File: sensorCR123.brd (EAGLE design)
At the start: 29.3 x 16.2 mm, 21 parts, among them IC1 LM75AD, IC4 RFM69, X1 16 MHz

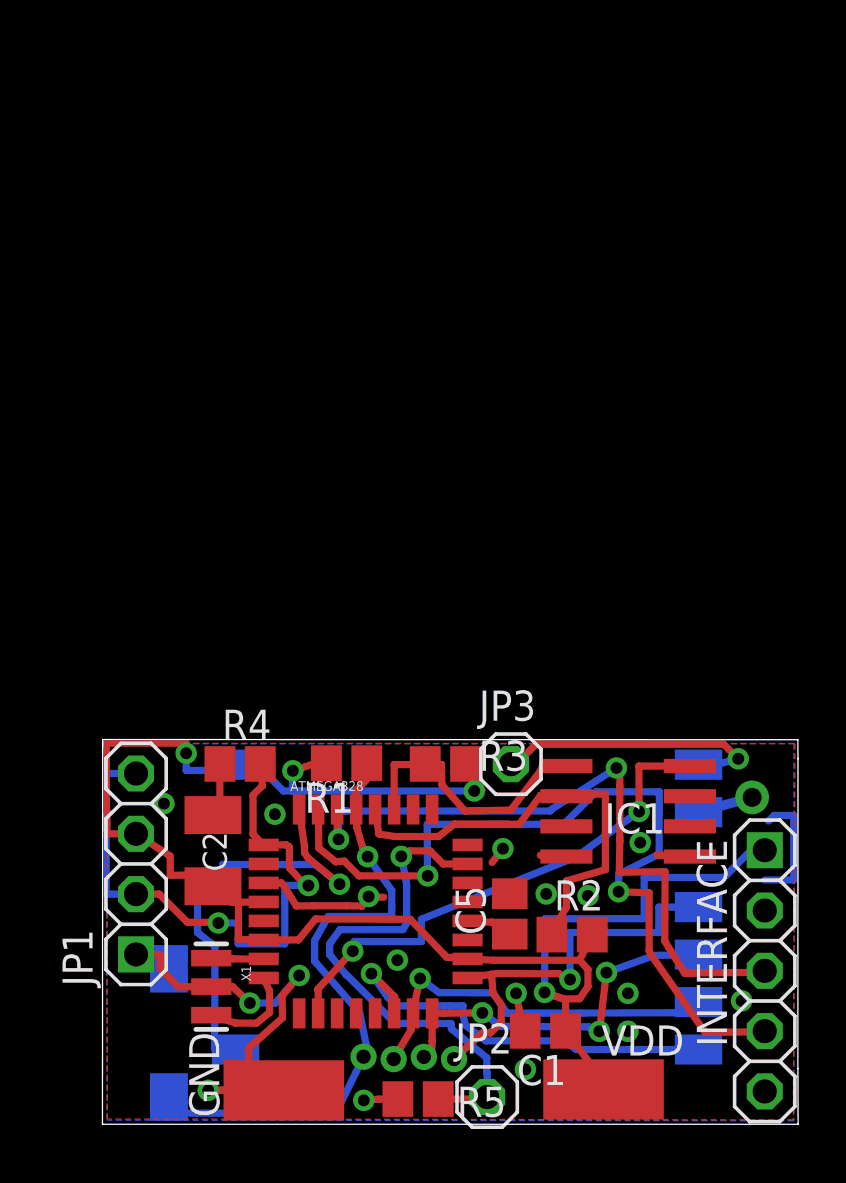
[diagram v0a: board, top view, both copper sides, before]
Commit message: Fixed bugs
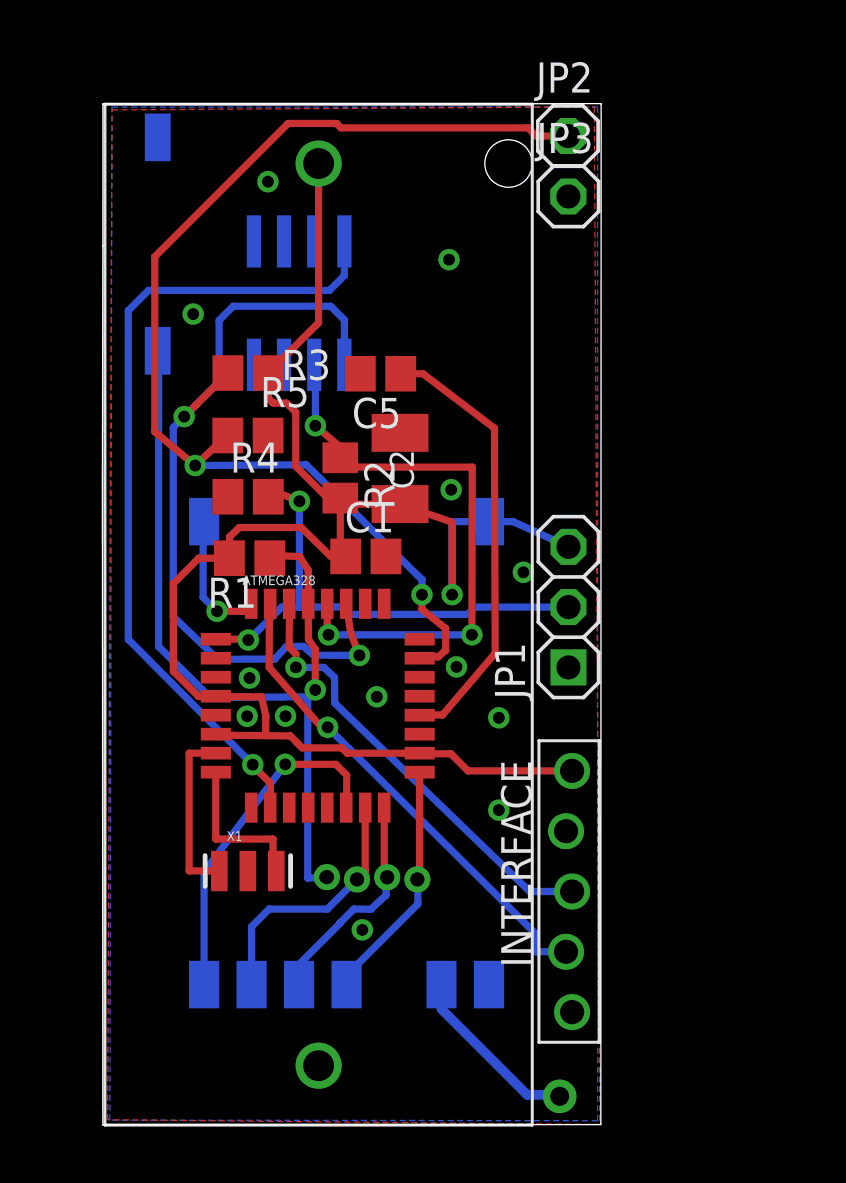
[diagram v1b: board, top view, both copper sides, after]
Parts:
- removed GND, VDD: (no value), wirepad:SMD2,54-5,08
- added U$3: BATT-CR123A, eagle-library-edeca.net-v5:KEYSTONE-2/3A
- INTERFACE: value (none) -> PINHD1X5SQUARE; device pinhead-2:1X05-S -> eagle-library-edeca.net-v5:PINHD1X05-SQUARE
- JP1: device pinhead-2:1X04-S -> pinhead-2:1X03-S
- RESET: device switch-tact:DTSM-3 -> smd-special:SMS-001
- moved JP2 40.6 mm to (19.6, 41.6)
- moved RESET 33.2 mm to (2.32, 37.1), turned to 0 degrees
- moved R5 28.9 mm to (6.12, 29.0), turned to 180 degrees
- moved IC1 25.5 mm to (8.27, 34.6), flipped to the bottom, turned to 0 degrees
- moved JP3 24.0 mm to (19.6, 39.1)
- moved C5 23.4 mm to (11.7, 31.6), turned to 180 degrees
- moved R2 21.6 mm to (10.0, 27.2), turned to 270 degrees
- moved C1 21.4 mm to (11.1, 23.9), turned to 0 degrees
- moved JP1 21.2 mm to (19.6, 21.8)
- moved R3 18.4 mm to (6.13, 31.6)
- moved C2 17.9 mm to (12.5, 27.6)
- moved U$1 15.0 mm to (19.3, 1.17)
- moved R4 11.3 mm to (6.13, 26.4)
- moved IC4 9.70 mm to (9.27, 13.9), turned to 270 degrees
- moved R1 9.55 mm to (6.19, 23.8)
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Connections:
- net D3: no longer JP1.4
- net GND: now also U$3.-VE; no longer GND.1
- net VCC: now also U$3.+VE; no longer VDD.1
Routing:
- net GND: track 52.7 -> 0.00 mm, vias 18 -> 13
- net A0: track 22.4 -> 47.6 mm, vias 1 -> 2
- net A4_SDA: track 12.4 -> 34.7 mm, vias 0 -> 2
- net AREF: track 2.09 -> 18.6 mm
- net D1_TX: track 34.9 -> 20.7 mm, vias 2 -> 1
- net D2: track 19.1 -> 5.61 mm
- net D6: track 21.7 -> 35.0 mm, vias 2 -> 1
- net D0_RX: track 29.6 -> 18.9 mm, vias 2 -> 1
- net RST: track 27.4 -> 35.8 mm, vias 1 -> 2
- net D13_SCK: track 17.6 -> 10.2 mm, vias 1 -> 0
- net VCC: track 77.2 -> 70.0 mm, vias 4 -> 1
- net D12_MISO: track 15.8 -> 9.55 mm, vias 3 -> 0
- net D11_MOSI: track 16.1 -> 10.9 mm, vias 1 -> 0
- net N$3: track 2.34 -> 7.53 mm
- net N$1: track 2.23 -> 7.36 mm
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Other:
- board size 29.3 x 16.2 mm -> 21 x 43 mm

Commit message: aaa
aaa
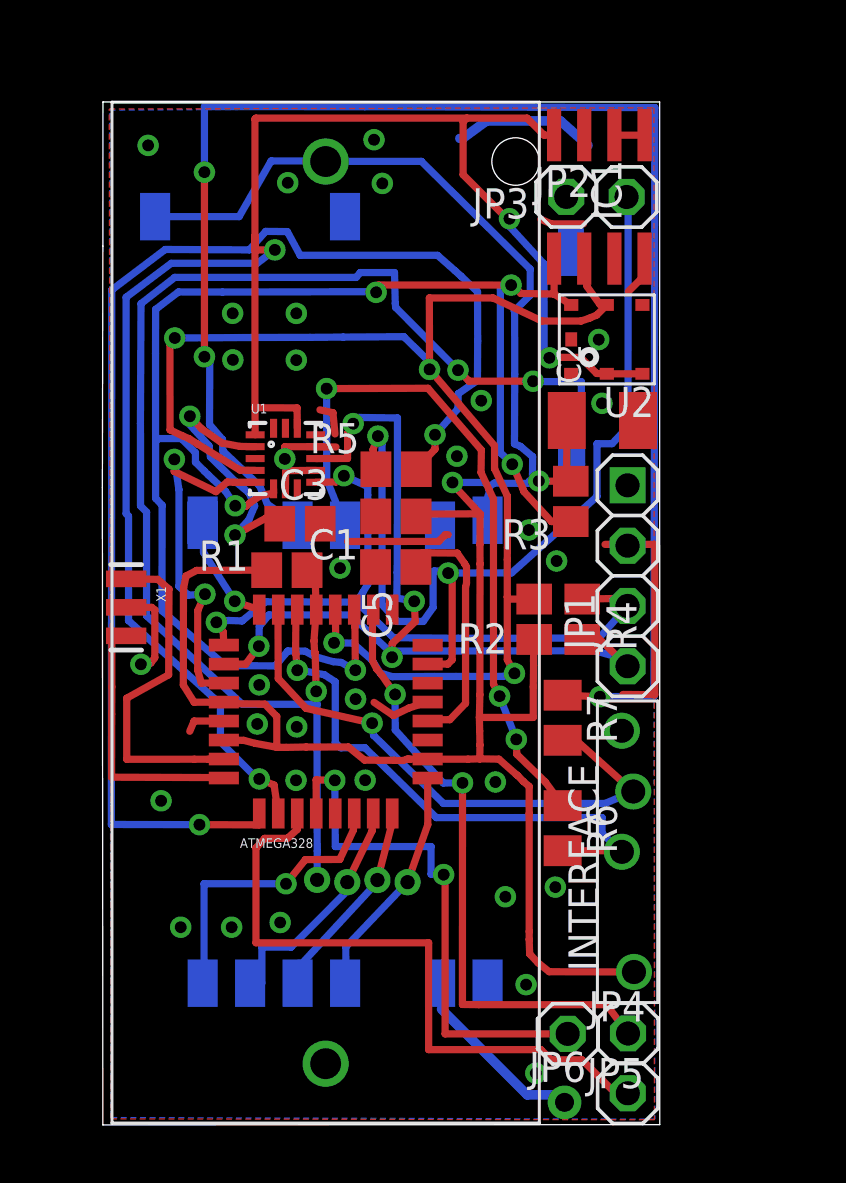
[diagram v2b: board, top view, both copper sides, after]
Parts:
- removed IC4: RFM69, LowPowerLab:RFM69W-MINPADS
- added C3: 100nF, resistor:C2012
- added JP4, JP5, JP6: (no value), pinhead-2:1X01
- added R6, R7: 1 K, resistor:M2012
- added U$4: RFM69W, RemoteHome:RFM69W
- added U$5: ESP03, RemoteHome:ESP03
- added U1: MMA8452Q, SparkFun-Sensors:QFN-16_0.5MM
- added U2: BMP180, SparkFun-Sensors:BMP180
- JP1: device pinhead-2:1X03-S -> pinhead-2:1X04-S
- moved RESET 18.1 mm to (19.7, 32.2)
- moved R4 15.0 mm to (20.2, 21.3), turned to 270 degrees
- moved R3 14.6 mm to (19.7, 26.2), turned to 90 degrees
- moved IC1 13.4 mm to (20.9, 39.1), flipped to the top
- moved X1 12.2 mm to (0.99, 21.8), turned to 270 degrees
- moved R2 10.1 mm to (18.2, 21.3)
- moved C2 8.76 mm to (21.0, 29.6), turned to 0 degrees
- moved C5 8.16 mm to (12.3, 23.5)
- moved R5 6.40 mm to (12.4, 27.6)
- moved JP2 3.56 mm to (22.1, 39.1)
- moved INTERFACE 2.98 mm to (22.1, 11.5), turned to 90 degrees
- moved JP1 2.82 mm to (22.1, 23.1), turned to 270 degrees
- moved C1 2.11 mm to (12.4, 25.6), turned to 180 degrees
- moved R1 1.65 mm to (7.76, 23.3)
- moved U$2 0.43 mm to (10.3, 10.2)
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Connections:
- new net N$10: R6.1, U$5.WIFI_TX
- new net N$11: R7.1, U$5.WIFI_RX
- new net N$2: C3.1, U1.2
- net A3: now also JP4.1
- net A4_SDA: now also U1.6, U2.6
- net A5_SCL: now also U1.4, U2.5
- net D0_RX: now also R6.2
- net D10_SS: now also U$4.NSS; no longer IC4.NSS
- net D11_MOSI: now also U$4.MOSI; no longer IC4.MOSI
- net D12_MISO: now also U$4.MISO; no longer IC4.MISO
- net D13_SCK: now also U$4.SCK; no longer IC4.SCK
- net D1_TX: now also R7.2
- net D2: now also U$4.DIO0, U$5.WIFI_EN; no longer IC4.DIO0
- net D3: now also JP1.3, R4.1, U1.9; no longer JP1.2, R4.2
- net D4: now also JP1.4, R4.2, U1.11
- net D5: now also R5.1
- net D6: now also U1.1, U1.14, U2.2, U2.3
- net D7: now also JP5.1
- net D8: now also JP6.1
- net GND: now also C3.2, JP1.2, U$4.GND, U$5.WIFI_GND, U$5.WIFI_GPIO15, U1.10, U1.12, U1.5, U1.7, U2.7; no longer IC4.GND, R4.1, R5.1
- net N$3: now also U$4.ANA; no longer IC4.ANA
- net VCC: now also U$4.VDD, U$5.WIFI_VDD; no longer IC4.VDD, JP1.3
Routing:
- net N$11: track 0.00 -> 66.9 mm, vias 0 -> 3
- net GND: track 0.00 -> 57.0 mm, vias 13 -> 34
- net D5: track 0.00 -> 55.3 mm, vias 0 -> 2
- net D6: track 35.0 -> 77.9 mm, vias 1 -> 4
- net D4: track 0.00 -> 37.9 mm, vias 0 -> 4
- net A5_SCL: track 24.5 -> 57.7 mm, vias 3 -> 4
- net N$10: track 0.00 -> 29.6 mm, vias 0 -> 3
- net VCC: track 70.0 -> 98.9 mm, vias 1 -> 2
- net A4_SDA: track 34.7 -> 63.3 mm, vias 2 -> 5
- net D7: track 0.00 -> 27.7 mm
- net A3: track 0.00 -> 26.1 mm, vias 0 -> 2
- net RST: track 35.8 -> 61.1 mm, vias 2 -> 3
- net D8: track 0.00 -> 22.7 mm, vias 0 -> 2
- net N$2: track 0.00 -> 11.7 mm, vias 0 -> 2
- net AREF: track 18.6 -> 10.5 mm
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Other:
- board size 21 x 43 mm -> 23.5 x 43.1 mm
